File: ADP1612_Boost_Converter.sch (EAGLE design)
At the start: 13 parts, among them U1 ADP1612ARMZ-R7D

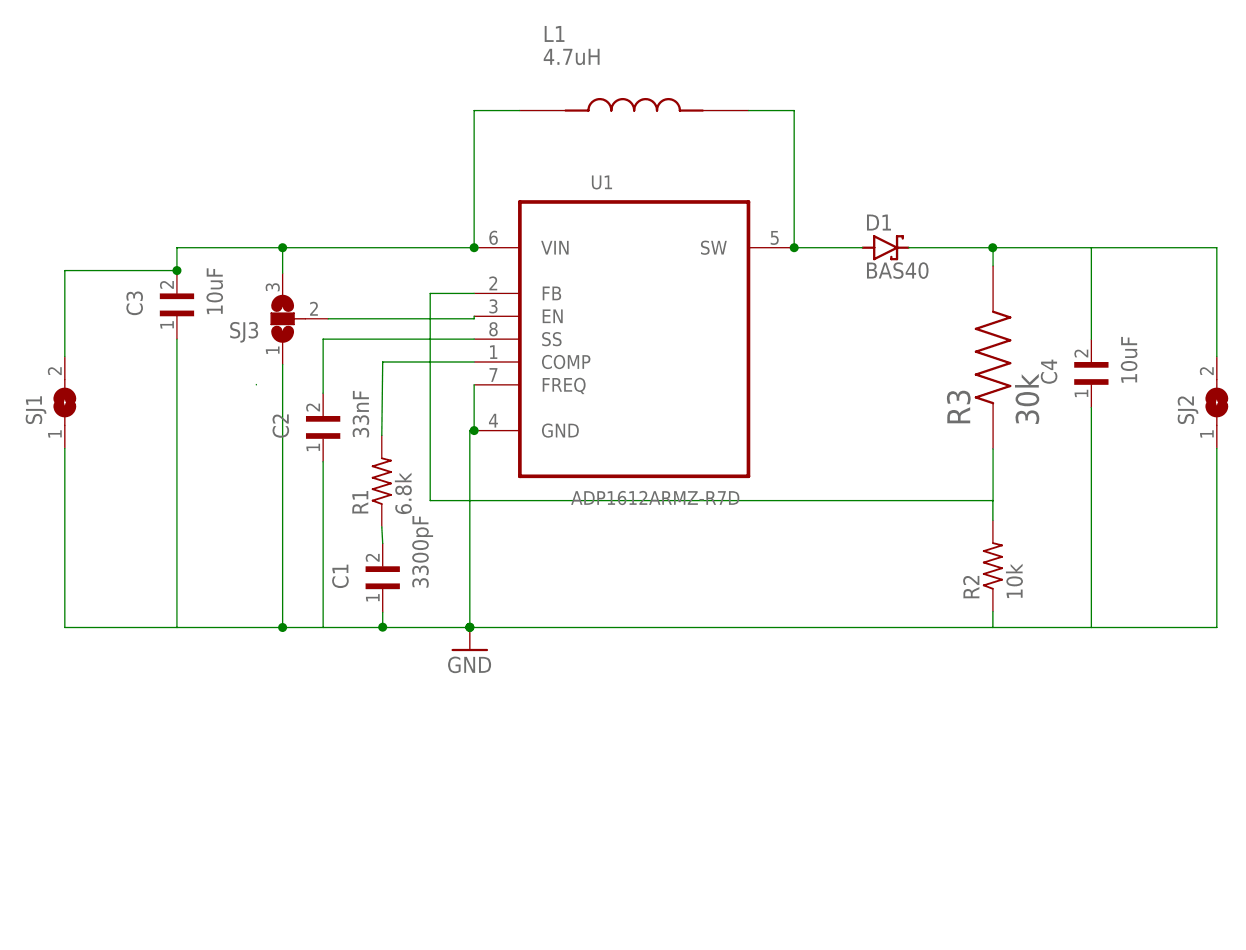
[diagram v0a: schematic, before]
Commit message: Add files via upload
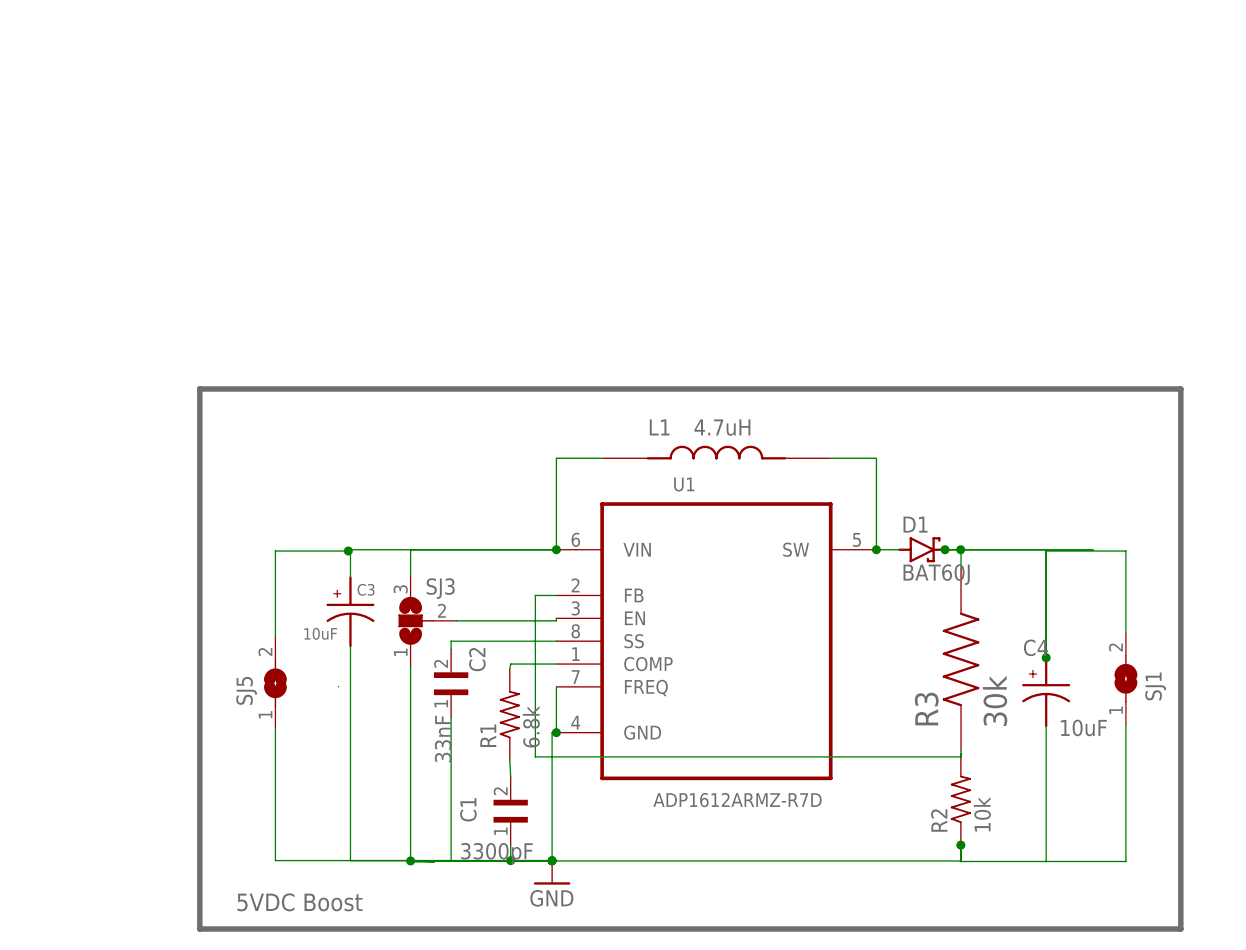
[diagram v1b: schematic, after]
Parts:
- removed SJ2: (no value), jumper:SJW
- added SJ5: (no value), jumper:SJW
- C3, C4: device Capacitor_10uF_smd_CAP-0135:GRM188C81C106MA73J -> EEE-1CA100SR_10uF_SMD:EEE-1CA100SR
- D1: value BAS40 -> BAT60J; device diode:BAS40 -> diode:BAT60J
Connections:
- removed net N$6: C4.2, D1.C, R3.2, SJ2.2
- removed net N$8: C3.2, L1.1, SJ1.2, SJ3.3, U1.VIN
- new net 5VDC: C4.1, D1.C, R3.2, SJ1.2
- new net N$1: C3.1, L1.1, SJ3.3, SJ5.2, U1.VIN
- net GND: now also C3.2, C4.2, SJ5.1; no longer C3.1, C4.1, SJ2.1
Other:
- note added: "5VDC Boost"
- moved on the sheet: C1, C2, C3, C4, L1, R1, R2, R3, SJ1, SJ3, U1
